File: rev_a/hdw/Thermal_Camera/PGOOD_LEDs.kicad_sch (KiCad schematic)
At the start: 5 parts, among them U1501 74LVC1G97

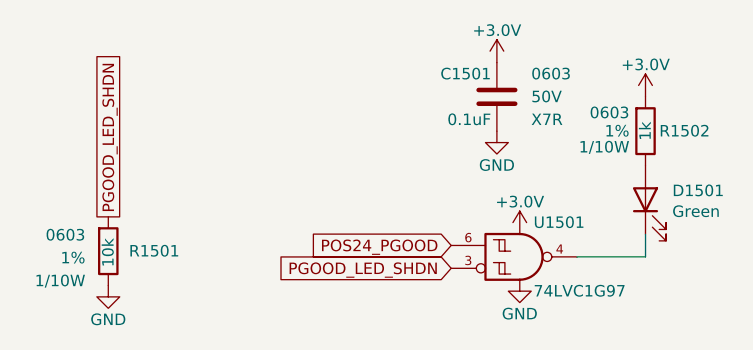
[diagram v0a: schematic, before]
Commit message: added some more USB stuff
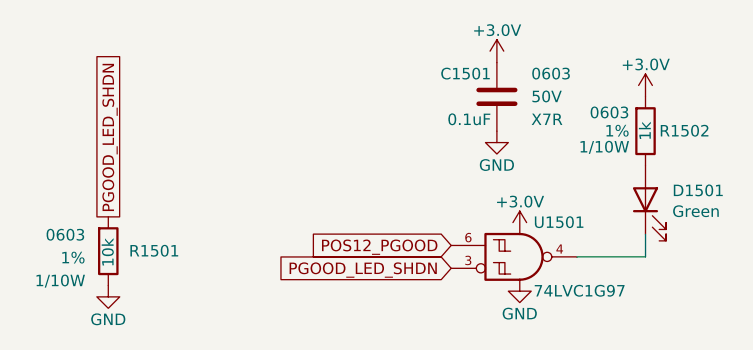
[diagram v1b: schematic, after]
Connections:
- net POS24_PGOOD renamed POS12_PGOOD
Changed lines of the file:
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@@
     )
   )
-  (global_label "POS24_PGOOD" (shape input) (at 64.77 55.88 180) (fields_autoplaced)
+  (global_label "POS12_PGOOD" (shape input) (at 64.77 55.88 180) (fields_autoplaced)
     (effects (font (size 1.27 1.27)) (justify right))
     (property "Intersheetrefs" "${INTERSHEET_REFS}" (at 48.1966 55.88 0)
